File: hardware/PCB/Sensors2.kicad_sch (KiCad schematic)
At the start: 25 parts, among them J12 Micro SD Adapter, J13 Relays, J14 Screw_Terminal_01x03, J201 Micro_SD_Card_Det2, J202 Screw_Terminal_01x03, J6 Screw_Terminal_01x03, K1 SANYOU_SRD_Form_C, K2 SANYOU_SRD_Form_C, K201 SANYOU_SRD_Form_C, Q1 NPN, Q201 NPN, Q3 NPN, U2 PC817C, U202 PC817C, U5 PC817C

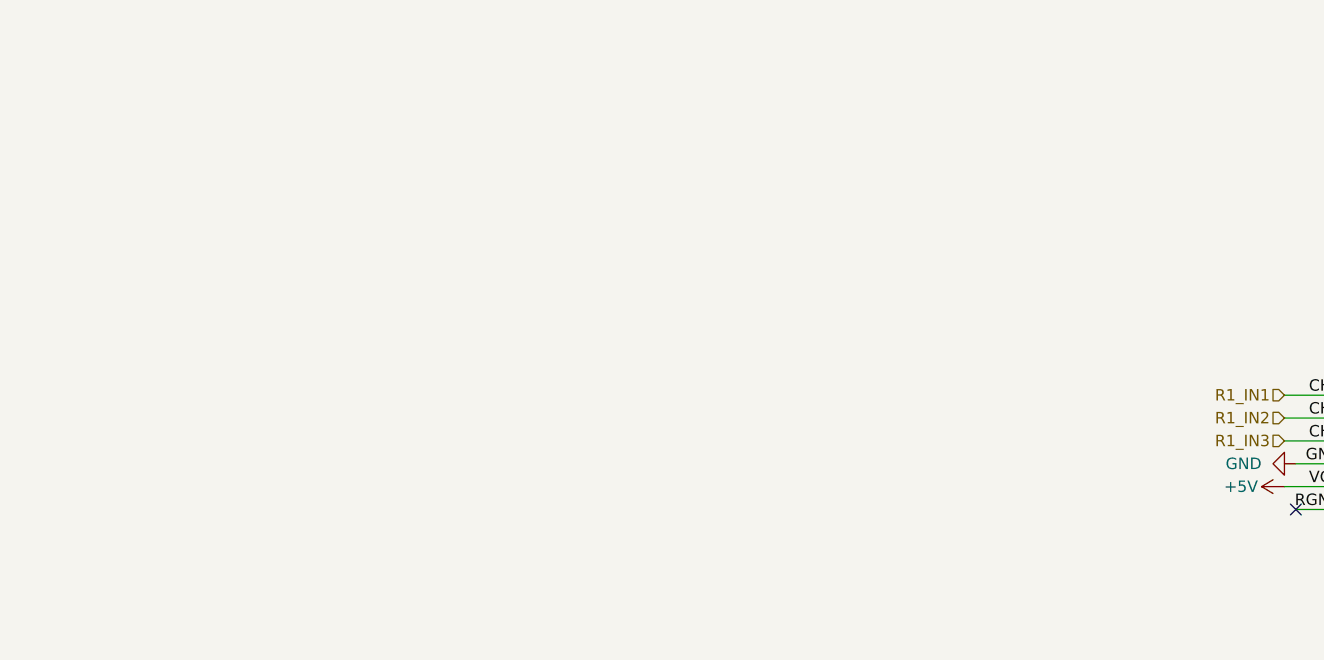
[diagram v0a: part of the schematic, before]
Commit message: PCB
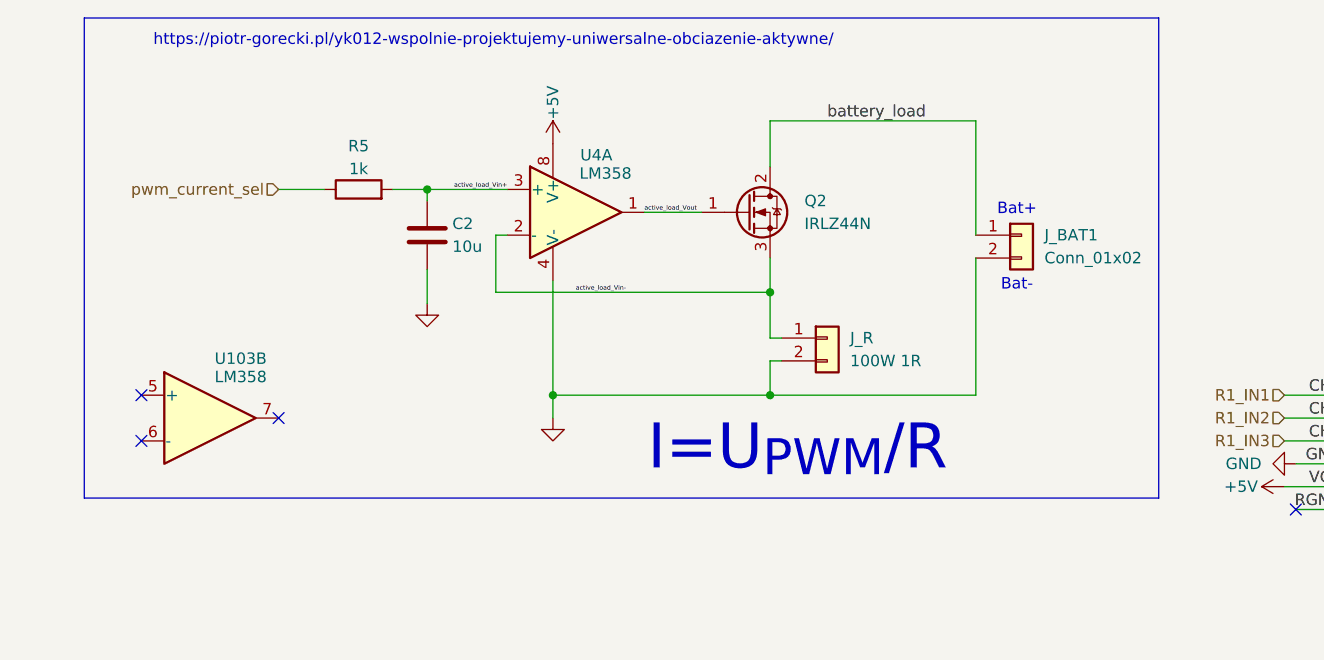
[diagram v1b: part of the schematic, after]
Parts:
- added C2: 10u, Capacitor_SMD:C_1206_3216Metric, symbol Device:C
- added J_BAT1: Conn_01x02, TerminalBlock:TerminalBlock_MaiXu_MX126-5.0-02P_1x02_P5.00mm, symbol Connector_Generic:Conn_01x02
- added J_R: 100W 1R, TerminalBlock:TerminalBlock_MaiXu_MX126-5.0-02P_1x02_P5.00mm, symbol Connector_Generic:Conn_01x02
- added Q2: IRLZ44N, Package_TO_SOT_THT:TO-220-3_Vertical, symbol Transistor_FET:IRLZ44N
- added R5: 1k, Resistor_SMD:R_0805_2012Metric, symbol Device:R
- added U103: LM358, footprints:LM358, symbol Amplifier_Operational:LM358
- added U4: LM358, Package_SO:SOIC-8_3.9x4.9mm_P1.27mm, symbol Amplifier_Operational:LM358
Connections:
- net +3V3: now also U4.8 (V+)
- net GND: now also C2.2, J_BAT1.2 (Pin_2), J_R.2 (Pin_2), U4.4 (V-)
- new net active_load_Vin+: C2.1, R5.2, U4.3 (+)
- new net active_load_Vin-: J_R.1 (Pin_1), Q2.3 (S), U4.2 (-)
- new net active_load_Vout: Q2.1 (G), U4.1
- new net battery_load: J_BAT1.1 (Pin_1), Q2.2 (D)
- new net pwm_current_sel: R5.1
- no-connect marks 1 -> 4
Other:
- note added: "Bat+"
- note added: "Bat-"
- note added: "I=U_{PWM}/R"
- note added: "https://piotr-gorecki.pl/yk012-wspolnie-projektujemy-uniwersalne-obciazenie-aktywne/"
